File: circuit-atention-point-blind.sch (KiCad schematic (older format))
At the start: 26 parts, among them IC1 STM8S003F3P, P1 RS485, P2 CON 4, P3 JSN-SR04T, U1 MAX485, U2 MC34063

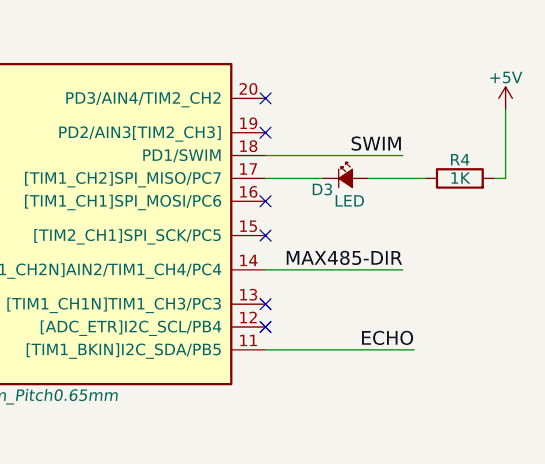
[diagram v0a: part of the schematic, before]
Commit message: backup PCB after modify 2nd
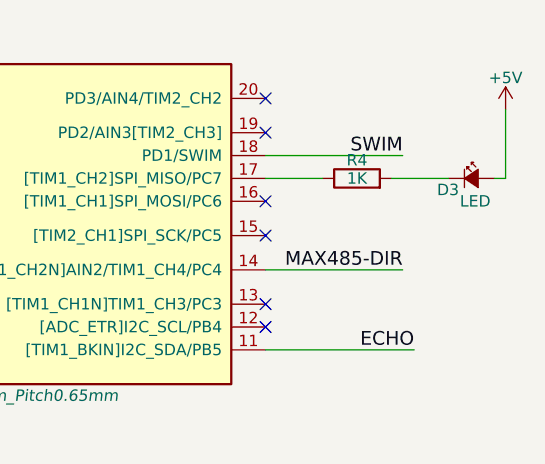
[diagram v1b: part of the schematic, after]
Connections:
- net +5V: now also D3.2 (A); no longer R4.2
- net at IC1.17 ([TIM1_CH2]SPI_MISO/PC7): now also R4.1; no longer D3.1 (K)
- new net: D3.1 (K), R4.2
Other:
- moved on the sheet: D3, R4
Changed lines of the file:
@@
 L R R4
 U 1 1 57772FB2
-P 9200 2450
-F 0 "R4" V 9280 2450 50  0000 C CNN
-F 1 "1K" V 9200 2450 50  0000 C CNN
-F 2 "Resistors_SMD:R_0805_HandSoldering" V 9130 2450 50  0001 C CNN
-F 3 "" H 9200 2450 50  0000 C CNN
-	1    9200 2450
+P 8750 2450
+F 0 "R4" V 8830 2450 50  0000 C CNN
+F 1 "1K" V 8750 2450 50  0000 C CNN
+F 2 "Resistors_SMD:R_0805_HandSoldering" V 8680 2450 50  0001 C CNN
+F 3 "" H 8750 2450 50  0000 C CNN
+	1    8750 2450
 	0    -1   -1   0
 $EndComp
@@
 L Led_Small D3
 U 1 1 577737B1
-P 8700 2450
-F 0 "D3" H 8550 2400 50  0000 L CNN
-F 1 "LED" H 8650 2350 50  0000 L CNN
-F 2 "LEDs:LED_0805" V 8700 2450 50  0001 C CNN
-F 3 "" V 8700 2450 50  0000 C CNN
-	1    8700 2450
+P 9250 2450
+F 0 "D3" H 9100 2400 50  0000 L CNN
+F 1 "LED" H 9200 2350 50  0000 L CNN
+F 2 "LEDs:LED_0805" V 9250 2450 50  0001 C CNN
+F 3 "" V 9250 2450 50  0000 C CNN
+	1    9250 2450
 	1    0    0    -1
 $EndComp
@@
 	1100 3700 1350 3700
 Wire Wire Line
-	8800 2450 9050 2450
+	8900 2450 9150 2450
 Wire Wire Line
 	8350 2350 8950 2350

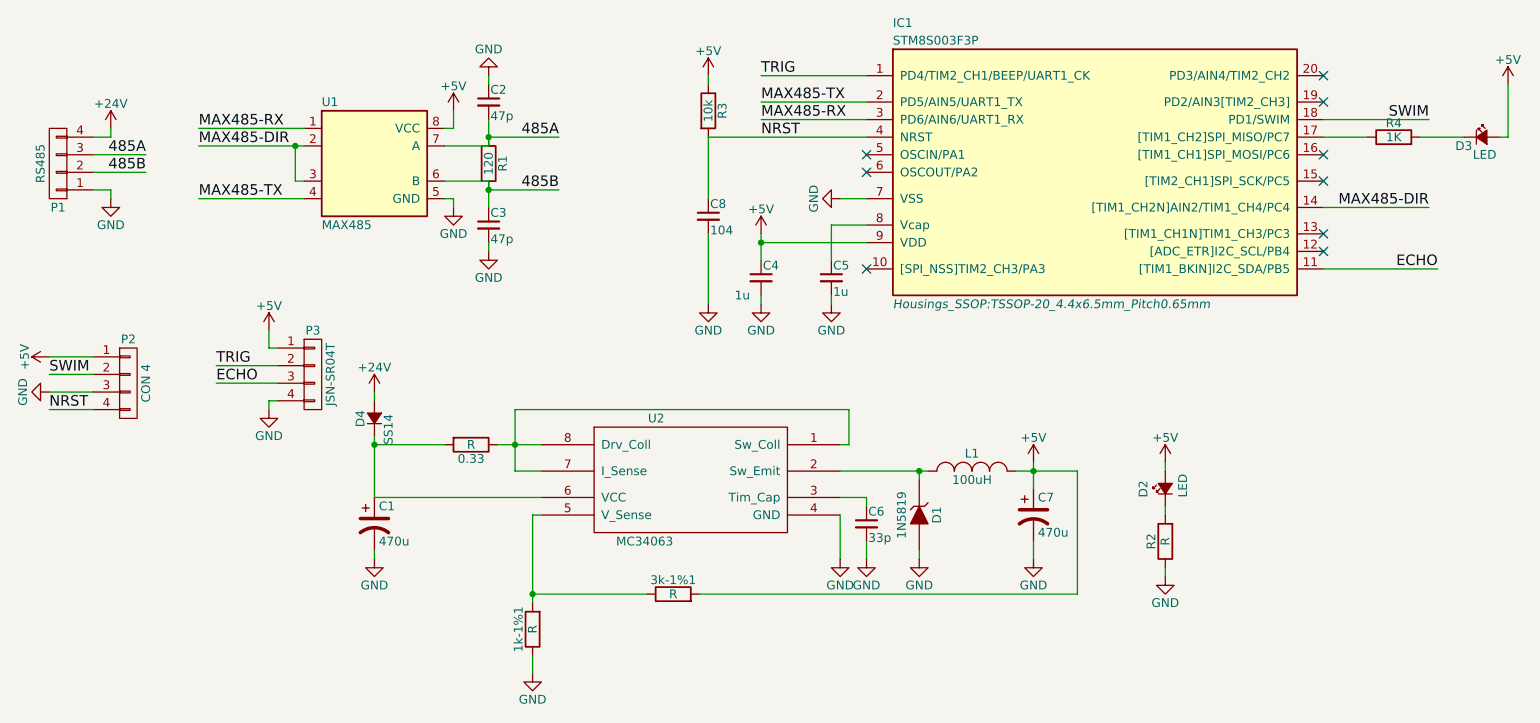
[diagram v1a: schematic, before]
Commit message: finish pcb (version1)
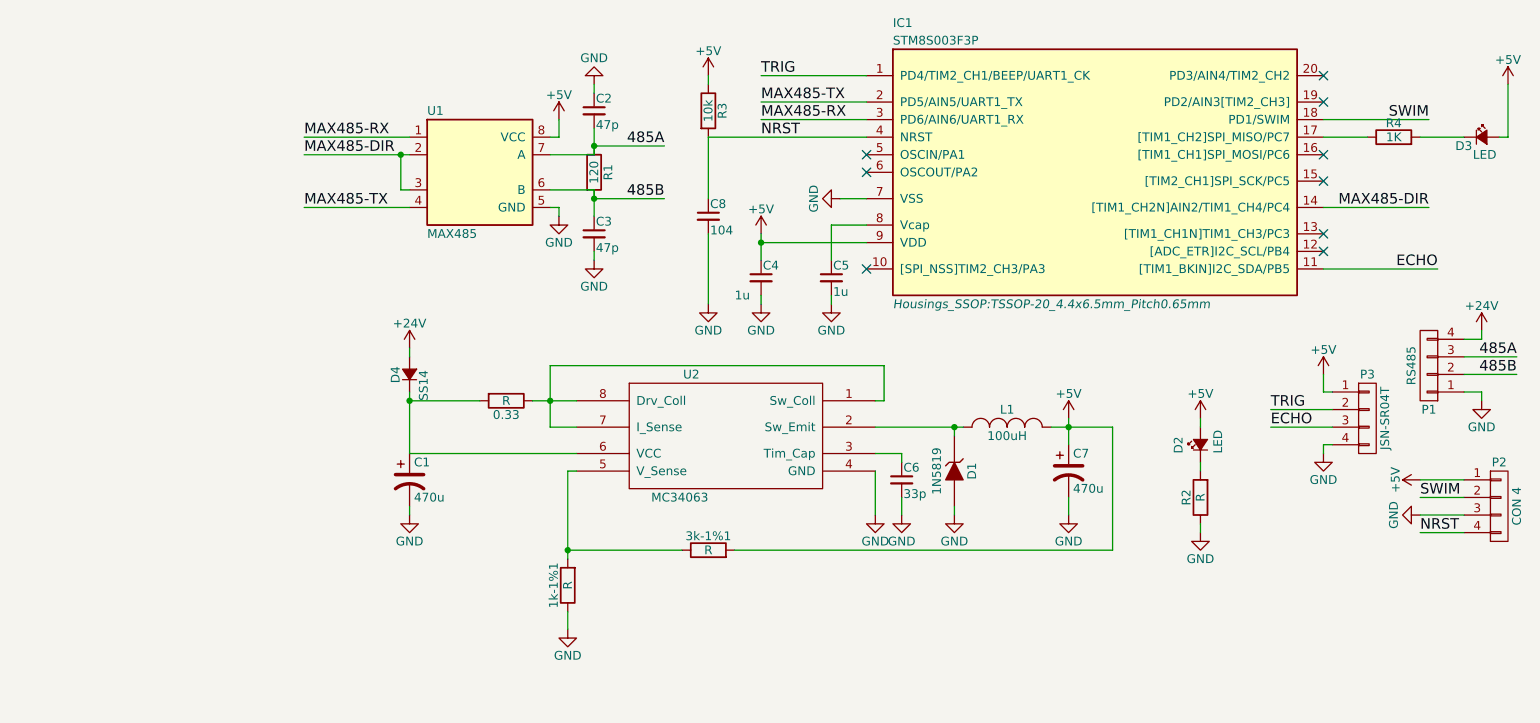
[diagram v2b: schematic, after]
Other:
- moved on the sheet: 0.33, 1k-1%1, 3k-1%1, C1, C2, C3, C6, C7, D1, D2, D4, L1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
